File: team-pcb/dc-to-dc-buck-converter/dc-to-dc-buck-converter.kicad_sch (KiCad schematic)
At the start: 11 parts, among them IC1 LM2596S-5.0_NOPB, J1 Screw_Terminal_01x02, J2 Screw_Terminal_01x02

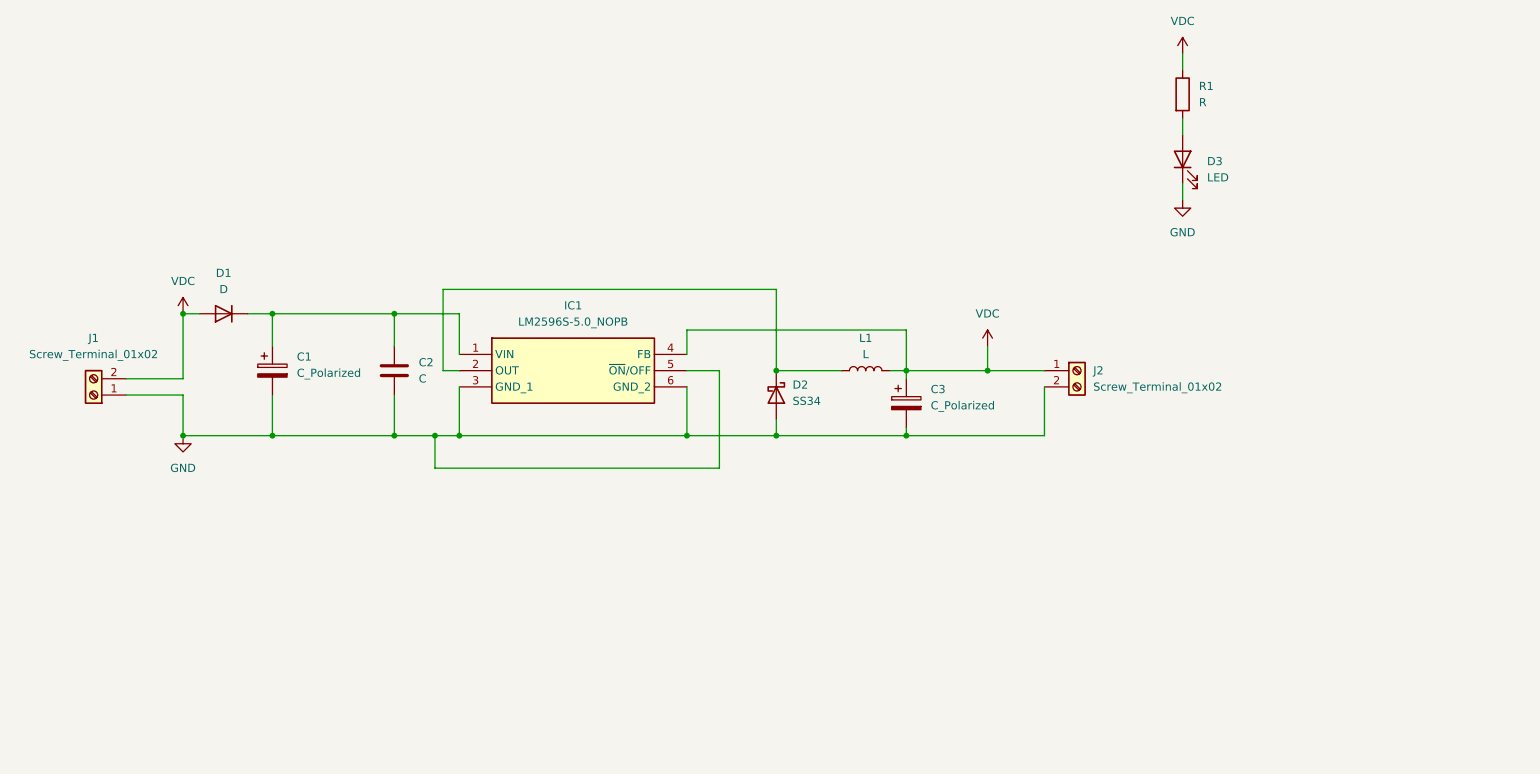
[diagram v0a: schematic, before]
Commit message: dc to dc
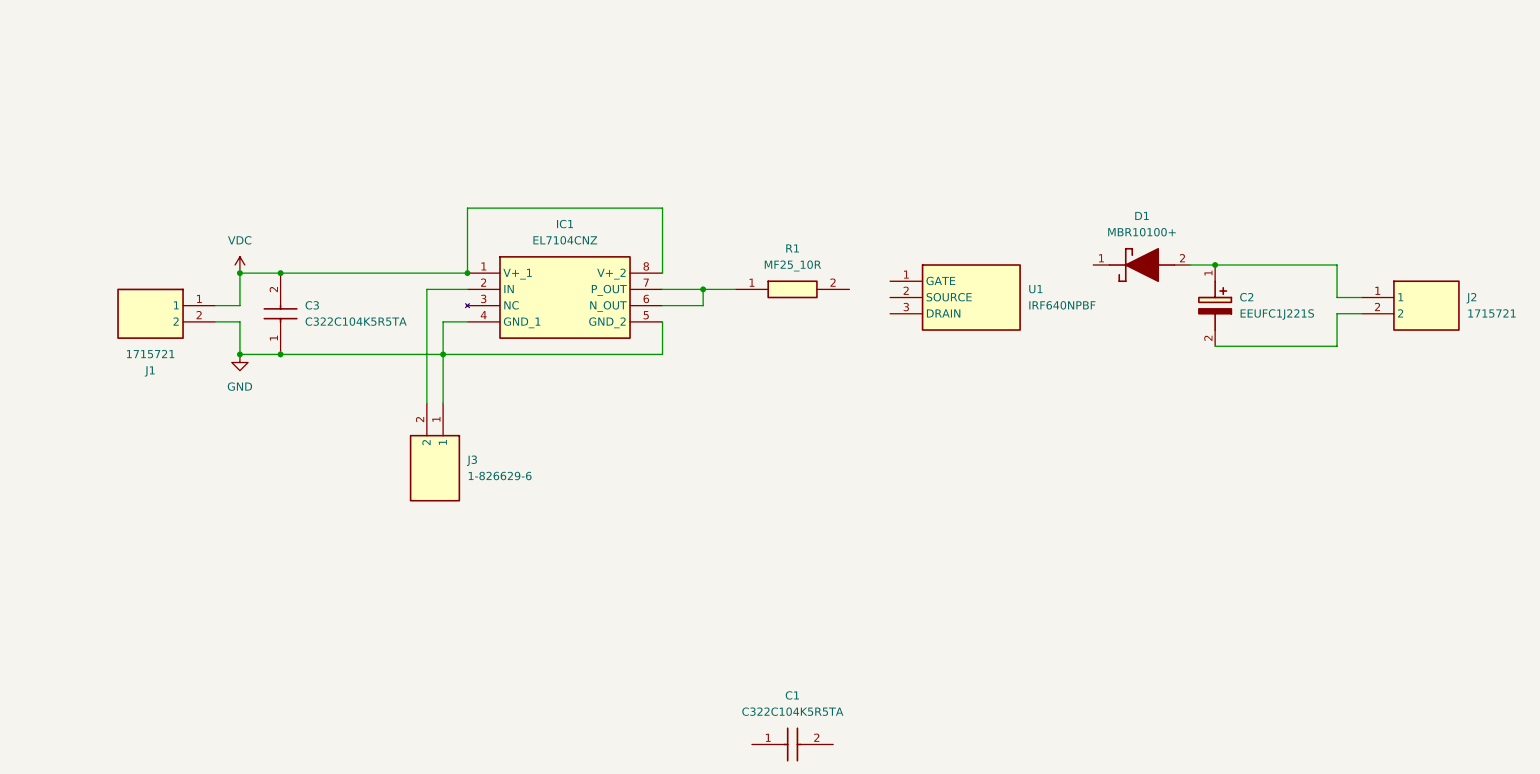
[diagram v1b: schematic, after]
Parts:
- removed C1, C3: C_Polarized, symbol Device:C_Polarized
- removed C2: C, symbol Device:C
- removed D1: D, symbol Device:D
- removed D2: SS34, Diode_SMD:D_SMA, symbol Diode:SS34
- removed D3: LED, symbol Device:LED
- removed IC1: LM2596S-5.0_NOPB, KTT0005B, symbol LM2596S-5_0_NOPB:LM2596S-5.0_NOPB
- removed J1, J2: Screw_Terminal_01x02, symbol Connector:Screw_Terminal_01x02
- removed L1: L, symbol Device:L
- removed R1: R, symbol Device:R
- added C1, C3: C322C104K5R5TA, C322C104K5R5TA(decoup capacitor):C322, symbol C322C104K5R5TA(decoup capacitor):C322C104K5R5TA
- added C2: EEUFC1J221S, EEUFC1J221S(capacitor):CAPPRD500W65D1250H2200, symbol EEUFC1J221S(capacitor):EEUFC1J221S
- added D1: MBR10100+, MBR10100+(diode):TO490P480X1000X2110-2P, symbol MBR10100+(diode):MBR10100+
- added IC1: EL7104CNZ, EL7104CNZ(voltage regulator):DIP762W51P254L952H533Q8N, symbol EL7104CNZ(voltage regulator):EL7104CNZ
- added J1, J2: 1715721, 1715721(screw connector):1715721, symbol 1715721(screw connector):1715721
- added J3: 1-826629-6, 1-826629-6(pins):HDRV16W63P0X254_1X16_4064X250X950P, symbol 1-826629-6(pins):1-826629-6
- added R1: MF25_10R, RESAD1680W59L680D250, symbol MF25_10R(resistor):MF25_10R
- added U1: IRF640NPBF, IRF640NPBF(mosfet):TO254P483X1016X1994-3P, symbol IRF640NPBF(mosfet):IRF640NPBF
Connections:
- net GND: now also C3.1, IC1.4 (GND_1), IC1.5 (GND_2), J1.2, J3.1
- net VDC: now also C3.2, IC1.1 (V+_1), IC1.8 (V+_2), J1.1
- new net: IC1.6 (N_OUT), IC1.7 (P_OUT), R1.1
- new net: IC1.2 (IN), J3.2
- new net: C2.1 (+), D1.2 (A), J2.1
- new net: C2.2 (-), J2.2
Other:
- company: (none) -> CBL Team 10
- title: (none) -> DC to DC Buck Boost Converter
